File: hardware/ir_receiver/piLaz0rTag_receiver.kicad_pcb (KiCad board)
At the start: 2 copper layers, 30 x 30 mm, 4 parts

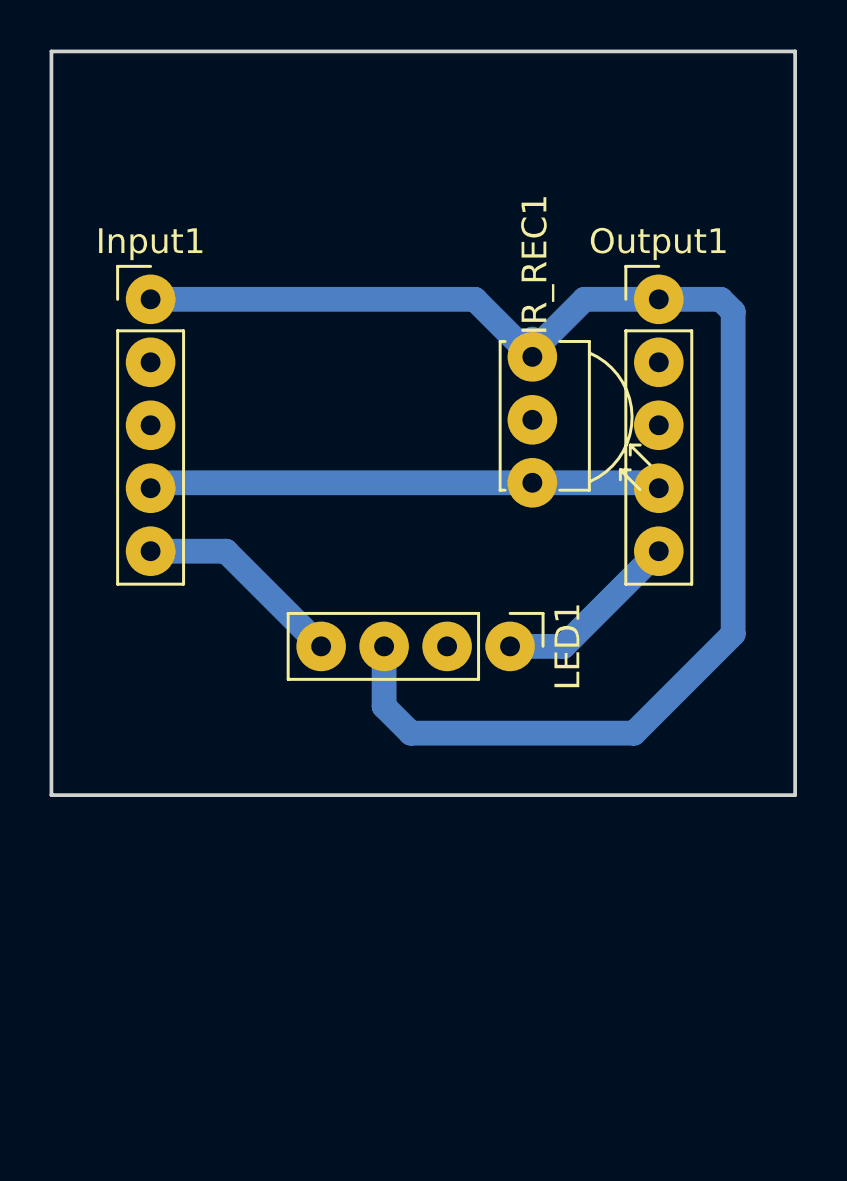
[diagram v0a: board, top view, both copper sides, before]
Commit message: Some rework on the receiver pcb
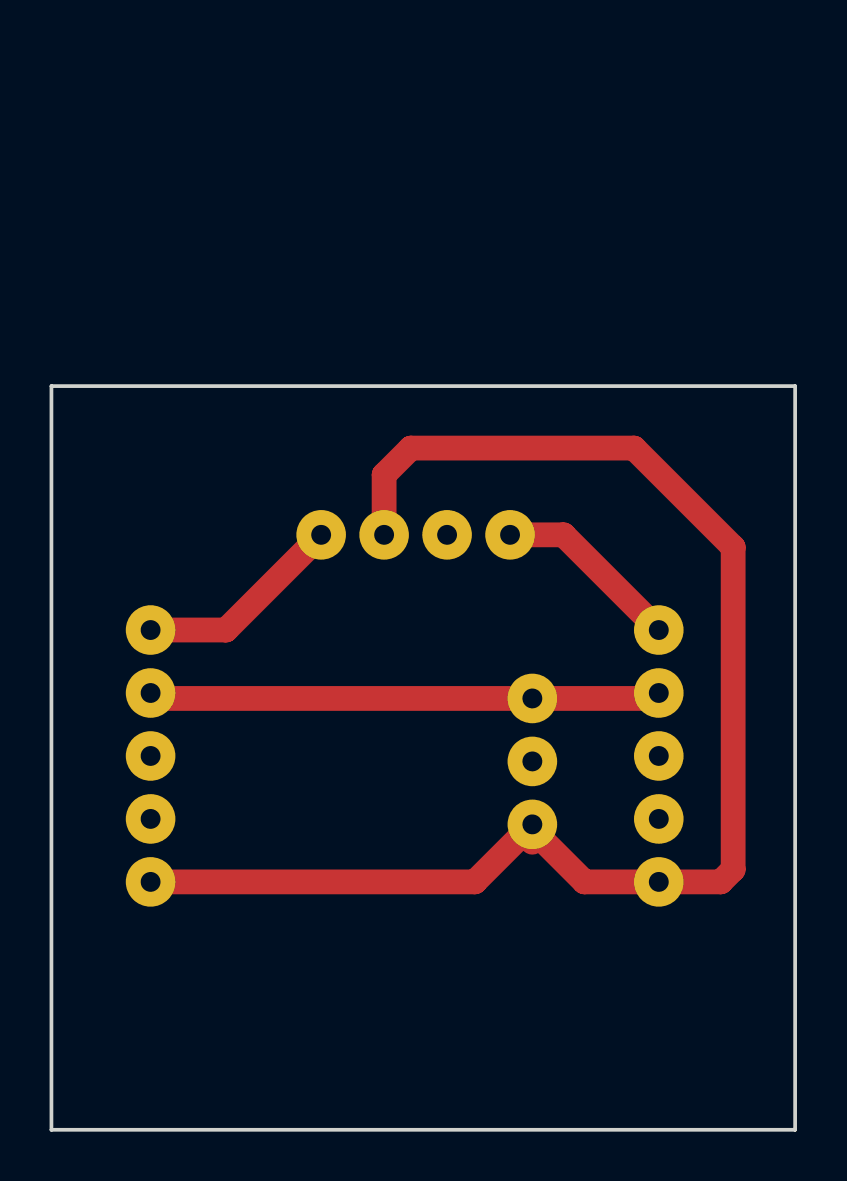
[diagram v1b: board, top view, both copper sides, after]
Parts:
- IR_REC1, Input1, LED1, Output1: moved to B.Cu
- moved Input1 23.5 mm to (94.0, 103.5)
- moved Output1 23.5 mm to (114.5, 103.5)
- moved IR_REC1 8.70 mm to (109.4, 96.1), turned to 270 degrees
- moved LED1 4.50 mm to (108.5, 89.5), turned to 90 degrees
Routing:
- added copper zone on F.Cu, net GND
- removed copper zone on B.Cu, net GND
